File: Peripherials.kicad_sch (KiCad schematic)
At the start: 24 parts, among them J6 Conn_01x02_Pin, J7 USB_C_Receptacle_USB2.0_14P, J8 USB_C_Receptacle_USB2.0_14P, Q1 NMOS, U5 USBLC6-2P6, U6 USBLC6-2P6

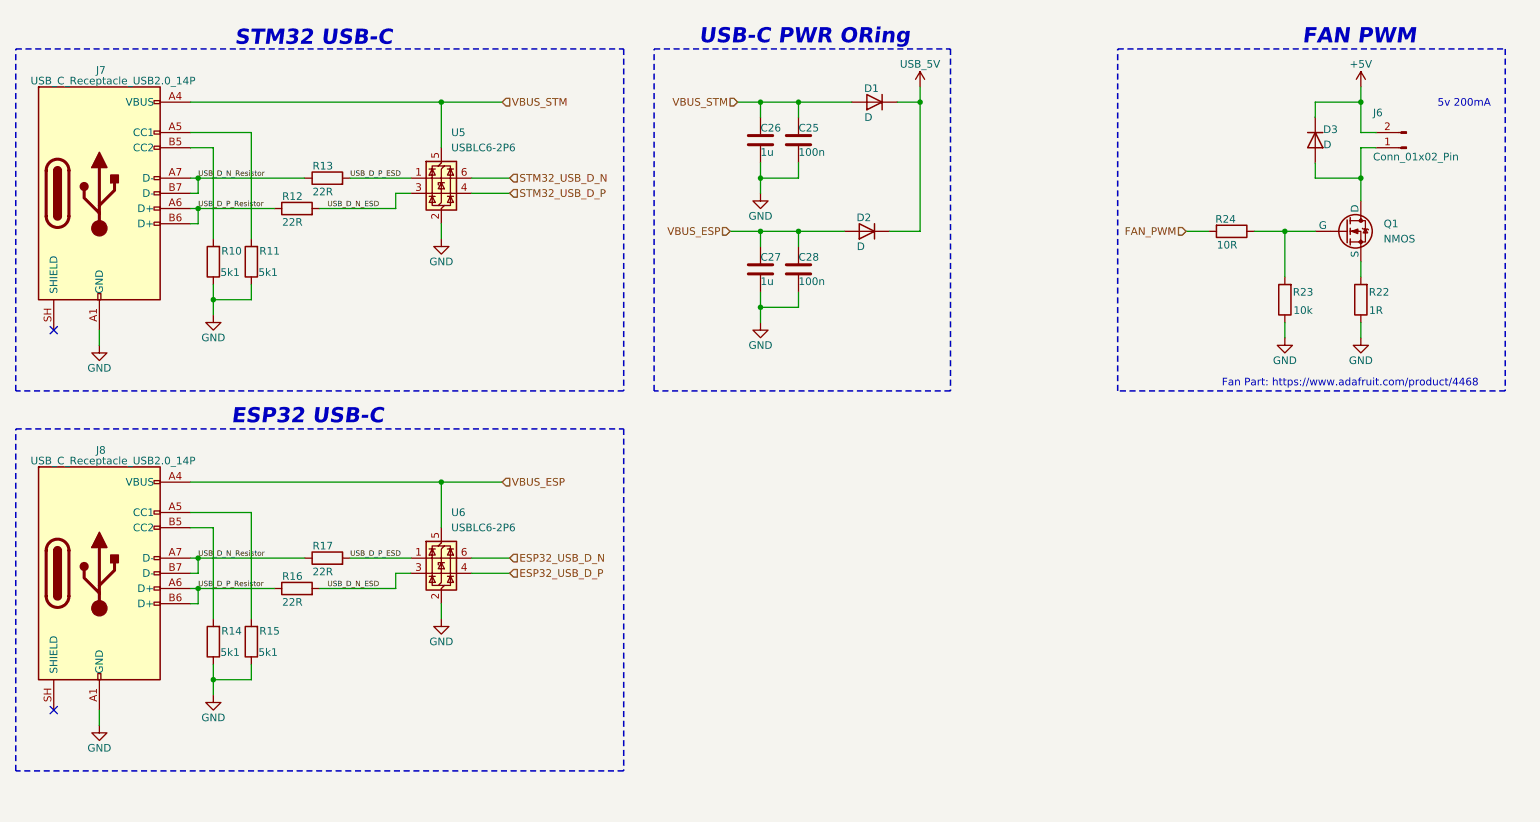
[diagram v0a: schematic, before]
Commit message: MIsc
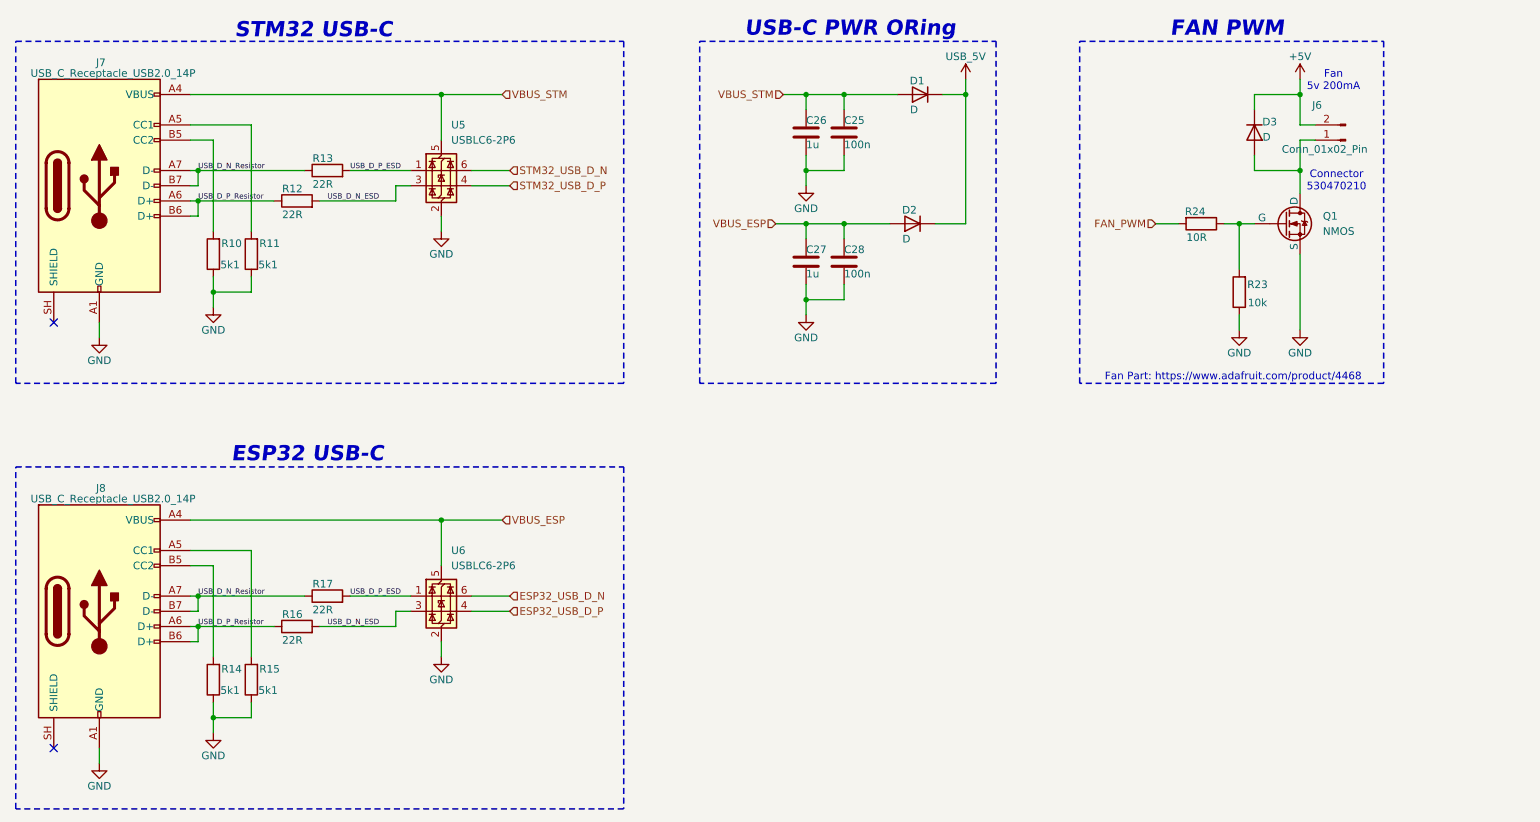
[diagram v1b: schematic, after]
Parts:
- removed R22: 1R, Package_DIP:DIP-8_W7.62mm, symbol Device:R
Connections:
- net GND: now also Q1.3 (S)
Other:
- note added: "Connector 530470210"
- note added: "Fan 5v 200mA"
- note removed: "5v 200mA"
- moved on the sheet: C25, C26, C27, C28, D1, D2, D3, J6, J7, J8, Q1, R10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
